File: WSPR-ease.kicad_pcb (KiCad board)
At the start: 4 copper layers, 100 x 75 mm, 98 parts, among them J101 GNSS Ant, J102 USB_C_16P_Stacked, J103 Tx Ant, Q101 MMBF170, Q102 MMBF170, Q103 MMBF170, Q104 MMBF170, Q105 MMBF170, Q106 MMBF170, Q107 MMBF170, Q108 MMBF170, Q109 MMBF170, Q110 MMBF170, Q111 MMBF170, Q112 MMBF170, SW101 BOOTSEL, SW102 RESET, T101 BN-43-202_DualPri_CTSec, U101 W25Q128JVS, U102 RP2040, U103 CD74AC244M, U104 ATGM336H-5N31, U105 NCP1117-3.3_SOT223, Y101 ABM8-272-T3

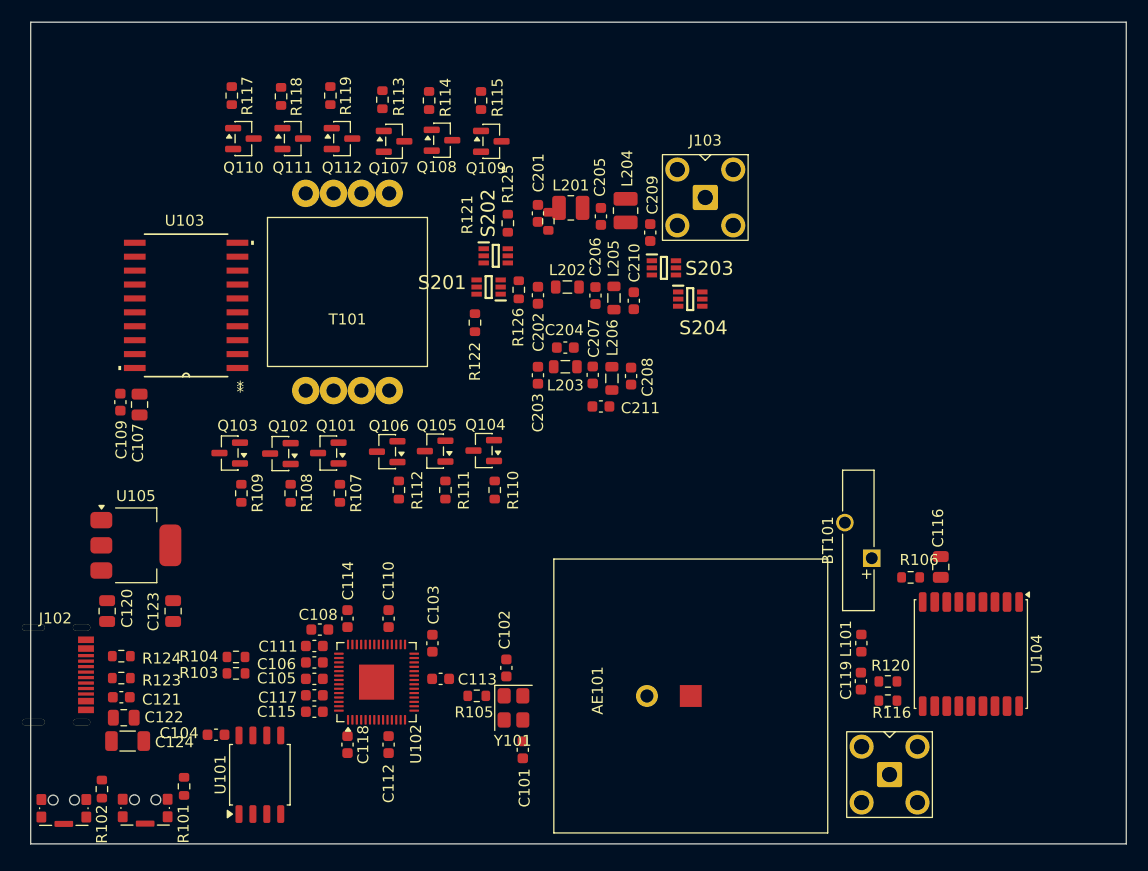
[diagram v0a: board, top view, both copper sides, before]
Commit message: Starting layout a bit
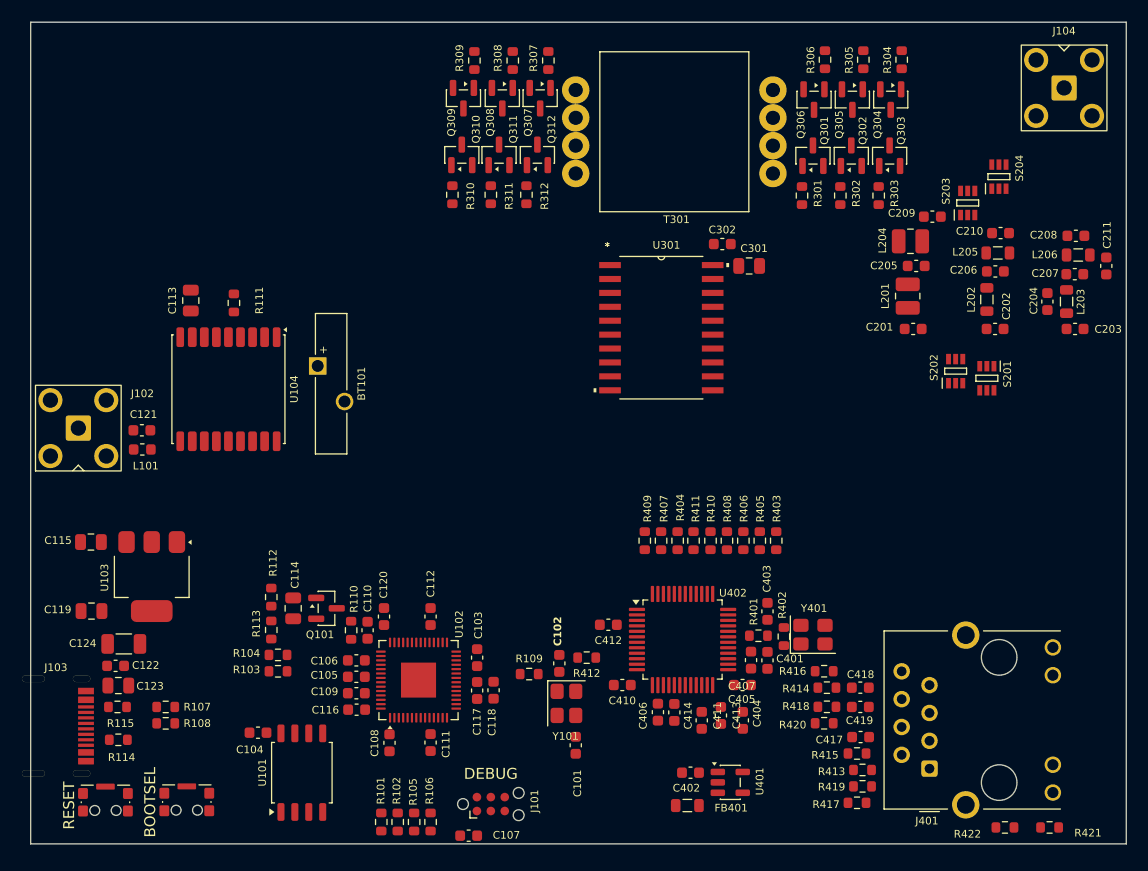
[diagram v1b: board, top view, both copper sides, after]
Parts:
- removed AE101: GPS_Patch_25mm, Library:gnss-antenna
- removed Q102, Q103, Q104, Q105, Q106, Q107, Q108, Q109, Q110, Q111, Q112: MMBF170, Package_TO_SOT_SMD:SOT-23
- removed R116, R120: 0, Resistor_SMD:R_0603_1608Metric
- removed R117, R118, R119: 10, Resistor_SMD:R_0603_1608Metric
- removed R121, R122, R125, R126: 100k, Resistor_SMD:R_0603_1608Metric
- removed R123, R124: 5.1k, Resistor_SMD:R_0603_1608Metric
- removed T101: BN-43-202_DualPri_CTSec, Library:bn-43-202-horizontal
- removed U105: NCP1117-3.3_SOT223, Package_TO_SOT_SMD:SOT-223-3_TabPin2
- added C301: 10uF, Capacitor_SMD:C_0805_2012Metric, F.Cu at (115.2, 80.7)
- added C302: 100nF, Capacitor_SMD:C_0603_1608Metric, F.Cu at (112.7, 78.7)
- added C401: 15pF, Capacitor_SMD:C_0603_1608Metric, F.Cu at (116.8, 116.7)
- added C402: 1uF, Capacitor_SMD:C_0603_1608Metric, F.Cu at (109.8, 126.9)
- added C403: 15pF, Capacitor_SMD:C_0603_1608Metric, F.Cu at (116.8, 112.2)
- added C404: 1uF, Capacitor_SMD:C_0603_1608Metric, F.Cu at (114.6, 122.1)
- added C405: 100nF, Capacitor_SMD:C_0603_1608Metric, F.Cu at (114.6, 118.9)
- added C406: 100nF, Capacitor_SMD:C_0603_1608Metric, F.Cu at (106.8, 121.4)
- added C407: 100nF, Capacitor_SMD:C_0603_1608Metric, F.Cu at (115.3, 116.6)
- added C410: 100nF, Capacitor_SMD:C_0603_1608Metric, F.Cu at (103.6, 118.9)
- added C411: 10nF, Capacitor_SMD:C_0603_1608Metric, F.Cu at (110.8, 122.1)
- added C412: 100nF, Capacitor_SMD:C_0603_1608Metric, F.Cu at (102.3, 113.4)
- added C413: 4.7uF, Capacitor_SMD:C_0603_1608Metric, F.Cu at (112.6, 121.7)
- added C414: 100nF, Capacitor_SMD:C_0603_1608Metric, F.Cu at (108.3, 121.4)
- added C417: 100nF, Capacitor_SMD:C_0603_1608Metric, F.Cu at (125.3, 123.7)
- added C418: 6.8nF, Capacitor_SMD:C_0603_1608Metric, F.Cu at (125.3, 119.1)
- added C419: 6.8nF, Capacitor_SMD:C_0603_1608Metric, F.Cu at (125.3, 120.9)
- added FB401: 120 @ 100MHz, Inductor_SMD:L_0805_2012Metric, F.Cu at (109.5, 129.9)
- added J104: Tx Ant, Connector_Coaxial:SMA_BAT_Wireless_BWSMA-KWE-Z001, F.Cu at (143.9, 64.4)
- added J401: RJ45_Hanrun_HR911105A_Horizontal, Connector_RJ:RJ45_Hanrun_HR911105A_Horizontal, F.Cu at (131.6, 126.5)
- added Q301: MMBF170, Package_TO_SOT_SMD:SOT-23, F.Cu at (121.0, 70.6)
- added Q302: MMBF170, Package_TO_SOT_SMD:SOT-23, F.Cu at (124.5, 70.6)
- added Q303: MMBF170, Package_TO_SOT_SMD:SOT-23, F.Cu at (128.0, 70.6)
- added Q304: MMBF170, Package_TO_SOT_SMD:SOT-23, F.Cu at (128.1, 65.5)
- added Q305: MMBF170, Package_TO_SOT_SMD:SOT-23, F.Cu at (124.6, 65.5)
- added Q306: MMBF170, Package_TO_SOT_SMD:SOT-23, F.Cu at (121.1, 65.5)
- added Q307: MMBF170, Package_TO_SOT_SMD:SOT-23, F.Cu at (96.1, 65.3)
- added Q308: MMBF170, Package_TO_SOT_SMD:SOT-23, F.Cu at (92.7, 65.3)
- added Q309: MMBF170, Package_TO_SOT_SMD:SOT-23, F.Cu at (89.1, 65.3)
- added Q310: MMBF170, Package_TO_SOT_SMD:SOT-23, F.Cu at (89.0, 70.5)
- added Q311: MMBF170, Package_TO_SOT_SMD:SOT-23, F.Cu at (92.3, 70.5)
- added Q312: MMBF170, Package_TO_SOT_SMD:SOT-23, F.Cu at (95.8, 70.5)
- added R301: 10, Resistor_SMD:R_0603_1608Metric, F.Cu at (120.0, 74.2)
- added R302: 10, Resistor_SMD:R_0603_1608Metric, F.Cu at (123.5, 74.2)
- added R303: 10, Resistor_SMD:R_0603_1608Metric, F.Cu at (127.0, 74.2)
- added R304: 10, Resistor_SMD:R_0603_1608Metric, F.Cu at (129.1, 61.8)
- added R305: 10, Resistor_SMD:R_0603_1608Metric, F.Cu at (125.6, 61.8)
- added R306: 10, Resistor_SMD:R_0603_1608Metric, F.Cu at (122.1, 61.8)
- added R307: 10, Resistor_SMD:R_0603_1608Metric, F.Cu at (96.8, 61.9)
- added R308: 10, Resistor_SMD:R_0603_1608Metric, F.Cu at (93.6, 61.9)
- added R309: 10, Resistor_SMD:R_0603_1608Metric, F.Cu at (90.1, 61.9)
- added R310: 10, Resistor_SMD:R_0603_1608Metric, F.Cu at (88.1, 74.2)
- added R311: 10, Resistor_SMD:R_0603_1608Metric, F.Cu at (91.6, 74.2)
- added R312: 10, Resistor_SMD:R_0603_1608Metric, F.Cu at (94.8, 74.2)
- added R401: 0, Resistor_SMD:R_0603_1608Metric, F.Cu at (116.0, 114.4)
- added R402: 1M, Resistor_SMD:R_0603_1608Metric, F.Cu at (118.3, 114.5)
- added R403: 10k, Resistor_SMD:R_0603_1608Metric, F.Cu at (117.7, 105.7)
- added R404: 10k, Resistor_SMD:R_0603_1608Metric, F.Cu at (108.7, 105.7)
- added R405: 10k, Resistor_SMD:R_0603_1608Metric, F.Cu at (116.2, 105.7)
- added R406: 10k, Resistor_SMD:R_0603_1608Metric, F.Cu at (114.7, 105.7)
- added R407: 10k, Resistor_SMD:R_0603_1608Metric, F.Cu at (107.1, 105.7)
- added R408: 10k, Resistor_SMD:R_0603_1608Metric, F.Cu at (113.2, 105.7)
- added R409: 10k, Resistor_SMD:R_0603_1608Metric, F.Cu at (105.7, 105.7)
- added R410: 10k, Resistor_SMD:R_0603_1608Metric, F.Cu at (111.7, 105.7)
- added R411: 10k, Resistor_SMD:R_0603_1608Metric, F.Cu at (110.1, 105.7)
- added R412: 12.4k, Resistor_SMD:R_0603_1608Metric, F.Cu at (100.3, 116.4)
- added R413: 3.3, Resistor_SMD:R_0603_1608Metric, F.Cu at (125.5, 126.7)
- added R414: 3.3, Resistor_SMD:R_0603_1608Metric, F.Cu at (122.3, 119.1)
- added R415: 49.9, Resistor_SMD:R_0603_1608Metric, F.Cu at (125.0, 125.2)
- added R416: 49.9, Resistor_SMD:R_0603_1608Metric, F.Cu at (122.0, 117.6)
- added R417: 49.9, Resistor_SMD:R_0603_1608Metric, F.Cu at (125.0, 129.7)
- added R418: 49.9, Resistor_SMD:R_0603_1608Metric, F.Cu at (122.0, 122.4)
- added R419: 3.3, Resistor_SMD:R_0603_1608Metric, F.Cu at (125.5, 128.2)
- added R420: 3.3, Resistor_SMD:R_0603_1608Metric, F.Cu at (122.3, 120.9)
- added R421: 1k, Resistor_SMD:R_0603_1608Metric, F.Cu at (142.6, 131.9)
- added R422: 1k, Resistor_SMD:R_0603_1608Metric, F.Cu at (138.5, 131.9)
- added T301: BN-43-202_DualPri_CTSec, Library:bn-43-202-horizontal, F.Cu at (108.3, 68.4)
- added U301: CD74AC244M, Library:DW20, F.Cu at (107.2, 86.3)
- added U401: LP5907MFX-3.3, Package_TO_SOT_SMD:SOT-23-5, F.Cu at (113.5, 127.8)
- added U402: W5500, Package_QFP:LQFP-48_7x7mm_P0.5mm, F.Cu at (109.1, 114.8)
- added Y401: 25MHz, Crystal:Crystal_SMD_Abracon_ABM8G-4Pin_3.2x2.5mm, F.Cu at (121.0, 114.3)
- C107: footprint Capacitor_SMD:C_0805_2012Metric -> Capacitor_SMD:C_0603_1608Metric
- C110: value 100nF -> 1uF
- C111: value 1uF -> 100nF
- C113, C115: value 100nF -> 10uF; footprint Capacitor_SMD:C_0603_1608Metric -> Capacitor_SMD:C_0805_2012Metric
- C114: footprint Capacitor_SMD:C_0603_1608Metric -> Capacitor_SMD:C_0805_2012Metric
- C116, C120, C122: value 10uF -> 100nF; footprint Capacitor_SMD:C_0805_2012Metric -> Capacitor_SMD:C_0603_1608Metric
- C119: value 100pF NP0 -> 10uF; footprint Capacitor_SMD:C_0603_1608Metric -> Capacitor_SMD:C_0805_2012Metric
- C121: value 100nF -> 100pF NP0
- J101: value GNSS Ant -> DEBUG; footprint Connector_Coaxial:SMA_BAT_Wireless_BWSMA-KWE-Z001 -> Connector:Tag-Connect_TC2030-IDC-NL_2x03_P1.27mm_Vertical
- J102: value USB_C_16P_Stacked -> GNSS Ant; footprint Library:HRO-TYPE-C-31-M-12 -> Connector_Coaxial:SMA_BAT_Wireless_BWSMA-KWE-Z001
- J103: value Tx Ant -> USB_C_16P_Stacked; footprint Connector_Coaxial:SMA_BAT_Wireless_BWSMA-KWE-Z001 -> Library:HRO-TYPE-C-31-M-12
- Q101: value MMBF170 -> 2N7002
- R101, R106: value 10k -> 100k
- R102, R105: value 1k -> 100k
- R103: value 27 -> 10k
- R104: value 27 -> 1k
- R107, R108: value 10 -> 27
- R109: value 10 -> 1k
- R110: value 10 -> 200
- R111: value 10 -> 10k
- R112: value 10 -> 200k
- R113: value 10 -> 100k
- R114, R115: value 10 -> 5.1k
- U103: value CD74AC244M -> NCP1117-3.3_SOT223; footprint Library:DW20 -> Package_TO_SOT_SMD:SOT-223-3_TabPin2
- Y101: value ABM8-272-T3 -> 12MHz
- moved J103 78.2 mm to (49.6, 122.7), turned to 90 degrees
- moved U104 72.0 mm to (67.7, 91.9)
- moved C119 70.5 mm to (55.1, 112.2), turned to 180 degrees
- moved L101 68.0 mm to (59.8, 97.4), turned to 180 degrees
- moved R114 64.9 mm to (57.6, 123.9), turned to 0 degrees
- moved R115 64.5 mm to (57.5, 120.9), turned to 0 degrees
- moved C116 54.9 mm to (79.3, 121.2), turned to 180 degrees
- moved BT101 53.5 mm to (75.8, 89.8), turned to -90 degrees
- moved C107 49.5 mm to (89.6, 132.7), turned to 180 degrees
- moved R113 49.5 mm to (71.6, 113.9), turned to -90 degrees
- moved C203 49.2 mm to (144.9, 86.4), turned to 0 degrees
- moved R106 49.2 mm to (86.1, 131.4), turned to -90 degrees
- moved C211 47.9 mm to (147.8, 80.7), turned to -90 degrees
- moved S201 46.2 mm to (136.9, 90.9), turned to -90 degrees
- moved L203 46.1 mm to (144.2, 83.9), turned to 90 degrees
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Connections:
- C107 pad 1: GND -> +3.3V
- C107 pad 2: +3.3V -> GND
- C109 pad 1: GND -> +3.3V
- C109 pad 2: +3.3V -> GND
- C110 pad 1: +3.3V -> Net-(U102-VREG_IN)
- C114 pad 1: +3.3V -> Net-(Q101-S)
- C115 pad 1: +3.3V -> VBUS
- C119 pad 1: Net-(C119-Pad1) -> +3.3V
- C119 pad 2: Net-(J101-In) -> GND
- C120 pad 1: VBUS -> +3.3V
- C121 pad 1: VBUS -> Net-(U104-RF_IN)
- C121 pad 2: GND -> Net-(J102-In)
- C123 pad 1: +3.3V -> VBUS
- J101 pad 1: Net-(J101-In) -> +3.3V
- J101 pad 2: GND -> /SWD
- L101 pad 2: Net-(J101-In) -> Net-(J102-In)
- Q101 pad 1: Net-(Q101-G) -> +3.3V
- Q101 pad 2: GND -> Net-(Q101-S)
- R101 pad 1: +3.3V -> /hiON
- R101 pad 2: Net-(U102-RUN) -> GND
- R102 pad 1: Net-(R102-Pad1) -> /loON
- R102 pad 2: /qsSS -> GND
- R103 pad 1: /D+ -> +3.3V
- R103 pad 2: Net-(U102-USB_DP) -> /nRESET
- R104 pad 1: /D- -> Net-(R104-Pad1)
- R104 pad 2: Net-(U102-USB_DM) -> /qsSS
- R105 pad 1: Net-(C102-Pad2) -> /lo1ON
- R105 pad 2: Net-(U102-XOUT) -> GND
- R106 pad 1: Net-(U102-GPIO14) -> /lo2ON
- R106 pad 2: /gnssPPS -> GND
- R107 pad 1: Net-(U103-1Y0) -> /D+
- R107 pad 2: Net-(Q101-G) -> Net-(U102-USB_DP)
- R108 pad 1: Net-(U103-1Y0) -> /D-
- R108 pad 2: Net-(Q102-G) -> Net-(U102-USB_DM)
- R109 pad 1: Net-(U103-1Y0) -> Net-(C102-Pad2)
- R109 pad 2: Net-(Q103-G) -> Net-(U102-XOUT)
- R110 pad 1: Net-(U103-1Y2) -> +3.3V
- R110 pad 2: Net-(Q104-G) -> Net-(U102-ADC_AVDD)
- R111 pad 1: Net-(U103-1Y2) -> Net-(U102-GPIO14)
- R111 pad 2: Net-(Q105-G) -> /gnssPPS
- R112 pad 1: Net-(U103-1Y2) -> VBUS
- R112 pad 2: Net-(Q106-G) -> Net-(Q101-S)
- R113 pad 1: Net-(U103-2Y0) -> Net-(Q101-S)
- R113 pad 2: Net-(Q107-G) -> GND
- R114 pad 1: Net-(U103-2Y0) -> Net-(J103-CC1)
- R114 pad 2: Net-(Q108-G) -> GND
- R115 pad 1: Net-(U103-2Y0) -> Net-(J103-CC2)
- R115 pad 2: Net-(Q109-G) -> GND
- SW101 pad 2: Net-(R102-Pad1) -> Net-(R104-Pad1)
- SW102 pad 2: Net-(U102-RUN) -> /nRESET
- U102 pad 24: unconnected-(U102-SWCLK-Pad24) -> /SWCLK
- U102 pad 25: unconnected-(U102-SWD-Pad25) -> /SWD
- U102 pad 26: Net-(U102-RUN) -> /nRESET
- U102 pad 27: unconnected-(U102-GPIO16-Pad27) -> /ethMISO
- U102 pad 28: unconnected-(U102-GPIO17-Pad28) -> /ethNCS
- U102 pad 29: unconnected-(U102-GPIO18-Pad29) -> /ethSCLK
- U102 pad 30: unconnected-(U102-GPIO19-Pad30) -> /ethMOSI
- U102 pad 31: unconnected-(U102-GPIO20-Pad31) -> /ethNIRQ
- U102 pad 32: unconnected-(U102-GPIO21-Pad32) -> /ethRESET
- U102 pad 41: unconnected-(U102-GPIO29_ADC3-Pad41) -> Net-(Q101-D)
- U102 pad 43: +3.3V -> Net-(U102-ADC_AVDD)
- U102 pad 44: +3.3V -> Net-(U102-VREG_IN)
- U103 pad 2: /push1 -> +3.3V
- U103 pad 3: Net-(U103-2Y2) -> VBUS
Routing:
- added copper zone on In2.Cu, net +3.3V
- added copper zone on In1.Cu, net GND
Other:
- board text added: "*"
